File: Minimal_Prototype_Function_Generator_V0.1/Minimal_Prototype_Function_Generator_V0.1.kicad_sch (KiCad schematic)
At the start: 3 parts, among them J13 142-0701-801

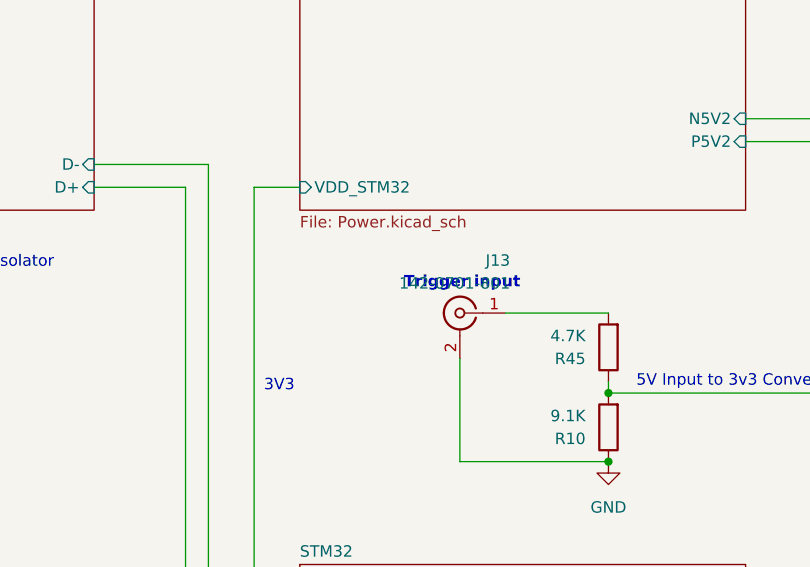
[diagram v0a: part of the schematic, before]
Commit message: V2.0
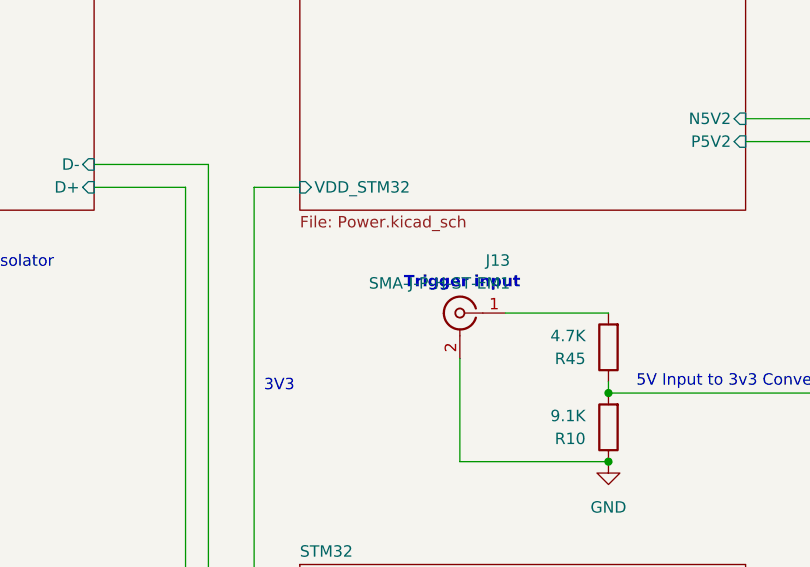
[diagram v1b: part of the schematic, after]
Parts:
- J13: value 142-0701-801 -> SMA-J-P-H-ST-EM1
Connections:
- net GND: no longer J13.4 (Ext), J13.5 (Ext)
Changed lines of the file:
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@@
 			)
 		)
-		(property "Value" "142-0701-801"
+		(property "Value" "SMA-J-P-H-ST-EM1"
 			(at 168.148 110.998 0)
 			(show_name no)
@@
 		(pin "3"
 		)
-		(pin "5"
-		)
-		(pin "4"
-		)
 		(instances
